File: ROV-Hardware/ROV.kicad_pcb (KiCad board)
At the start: 2 copper layers, 104 x 104 mm, 32 parts, among them J1 T-block, J2 T-block, J3 Screw_Terminal_01x04, SW1 switch, U1 LM7812, U2 LM7805, U3 ESP32-S3-DEVKITC-1-N8R2, U4 MPU6050, U5 ZK-BM1, U6 ZK-BM1, U7 ZK-BM1, U8 A4988, U9 GY-MS5837

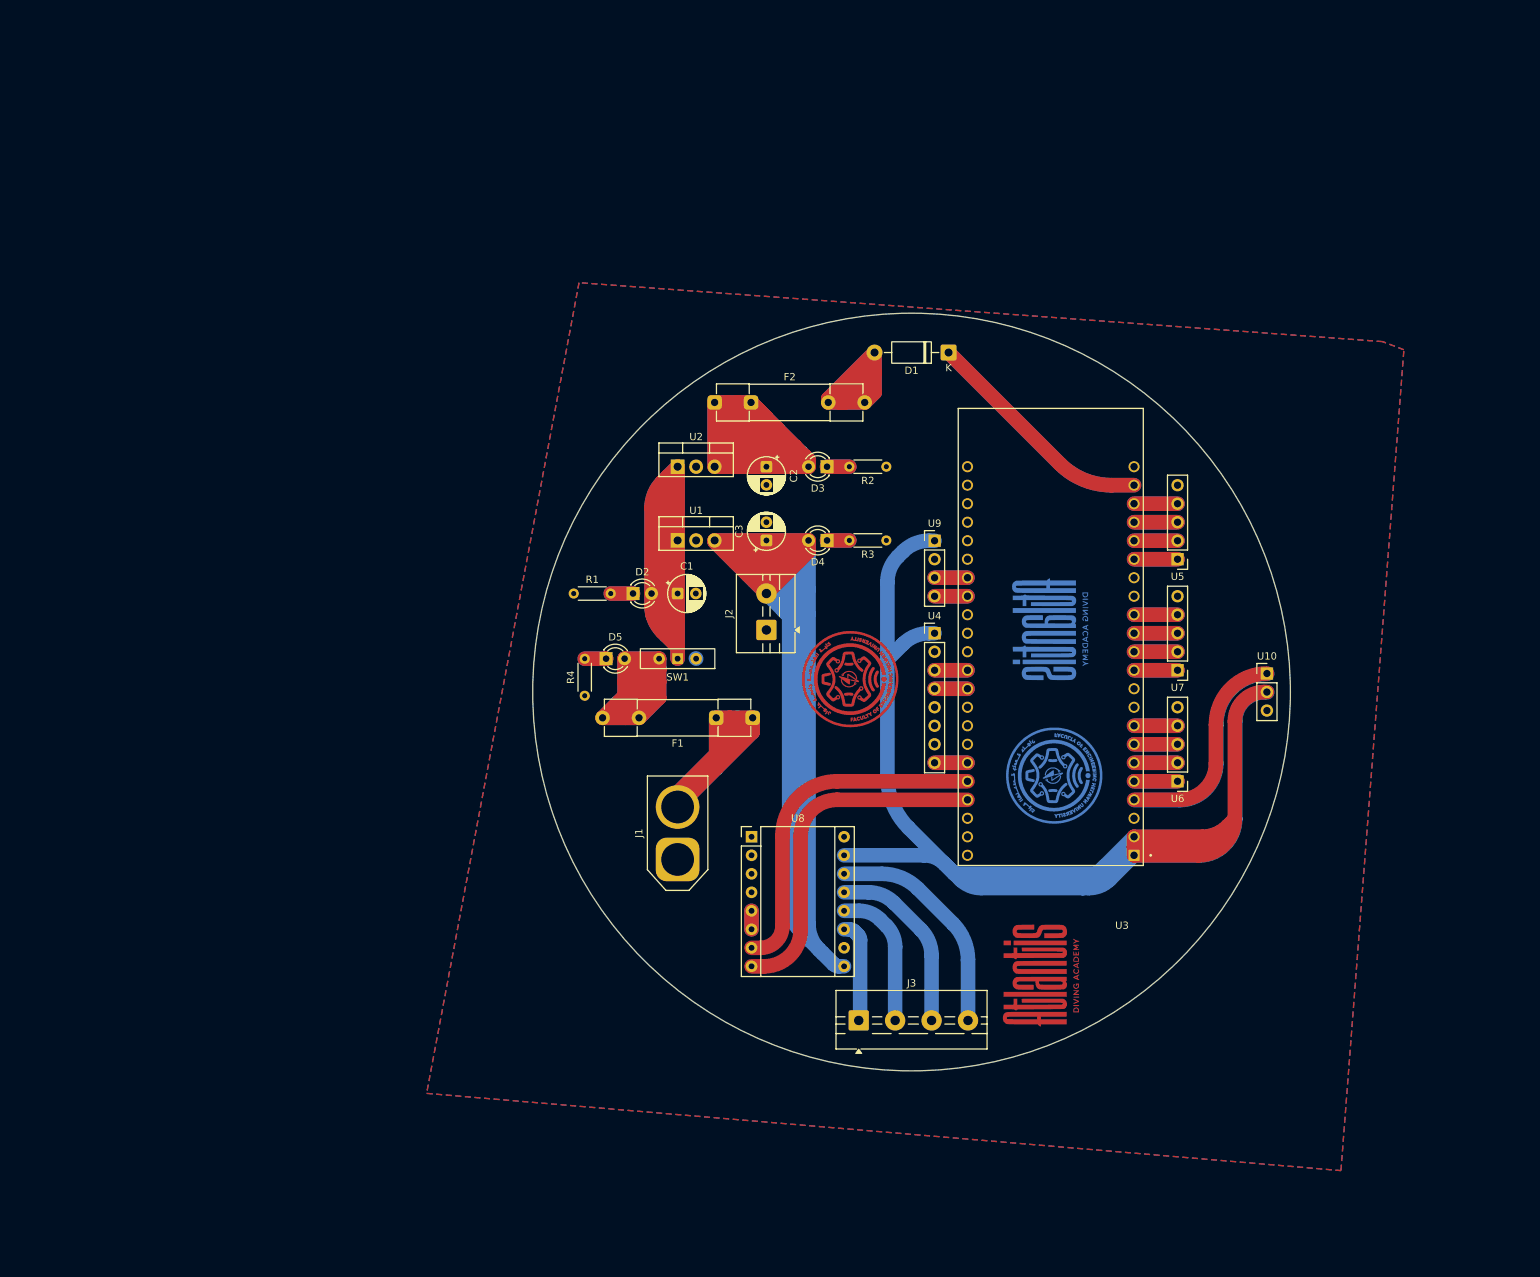
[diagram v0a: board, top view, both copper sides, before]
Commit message: hight current
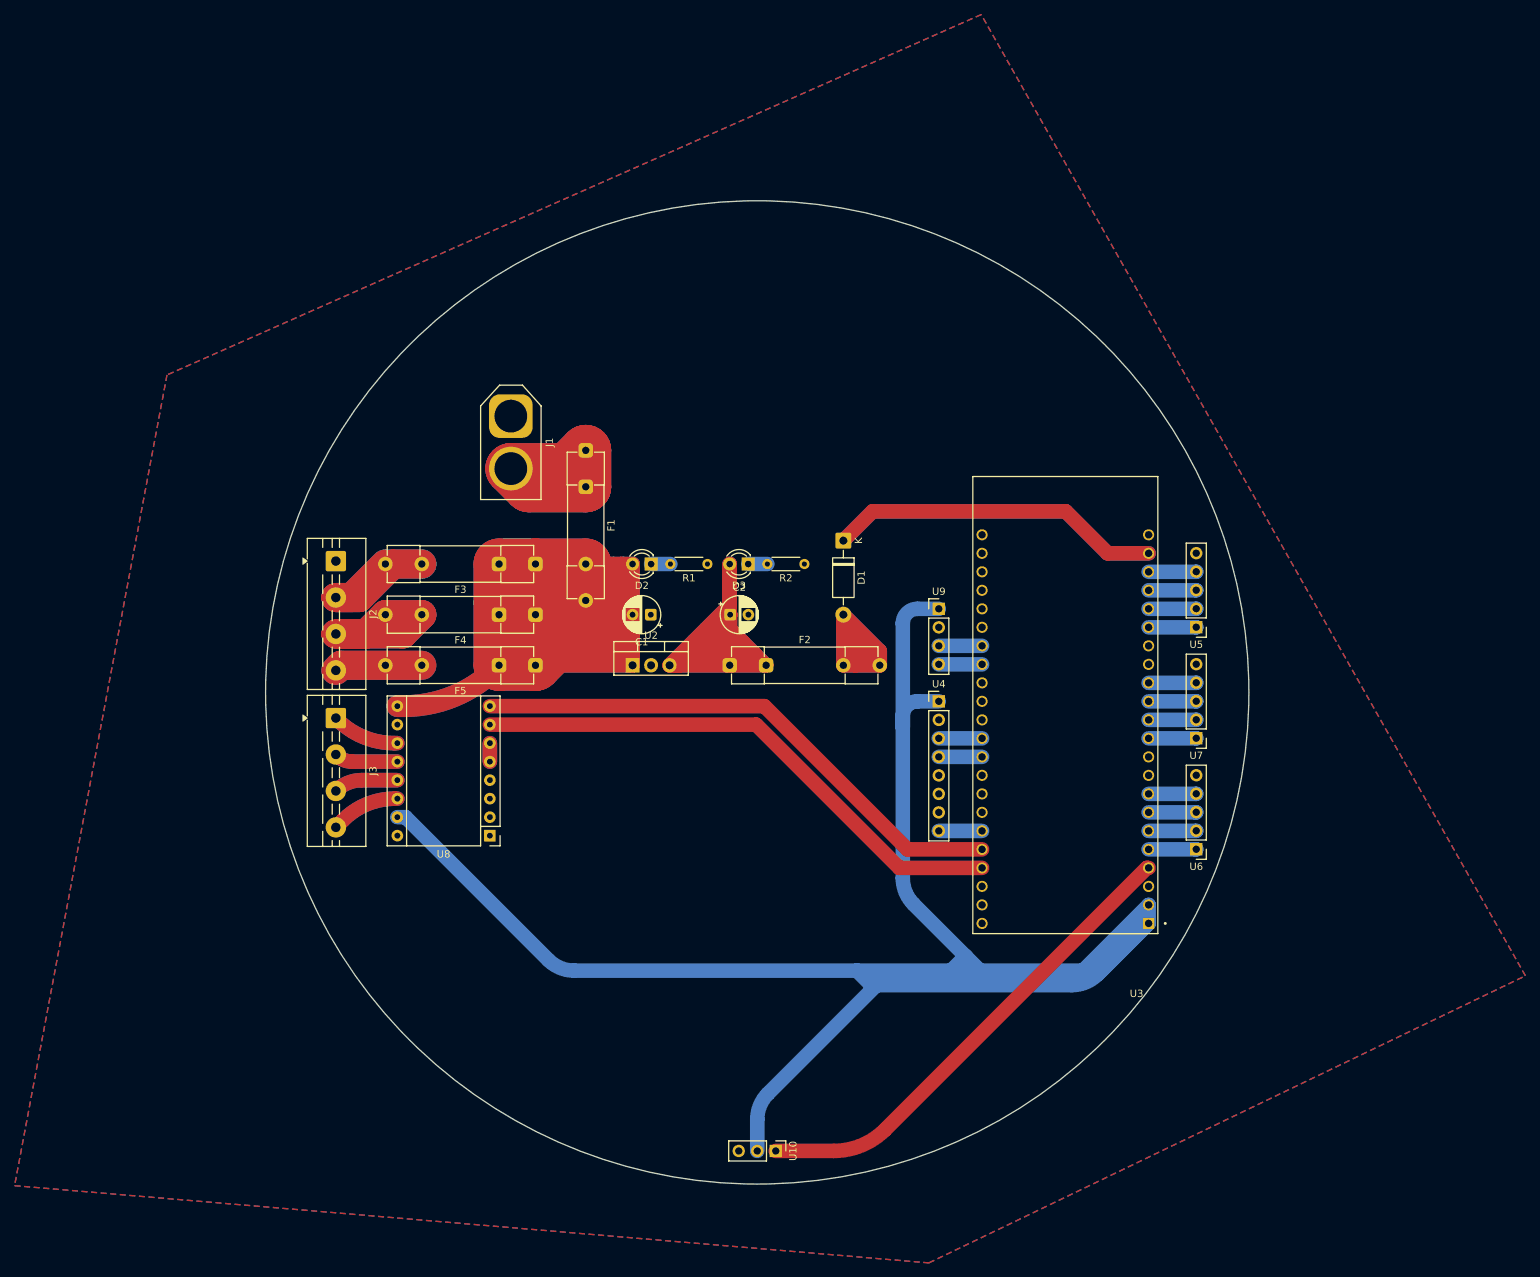
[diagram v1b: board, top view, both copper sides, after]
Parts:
- removed C3: capacitor, Capacitor_THT:CP_Radial_D5.0mm_P2.50mm
- removed D4, D5: LED, LED_THT:LED_D3.0mm
- removed G*** (x2): LOGO, logo:englogo4
- removed G*** (x2): LOGO, logo:logo7
- removed R3, R4: R, Resistor_THT:R_Axial_DIN0204_L3.6mm_D1.6mm_P5.08mm_Horizontal
- removed SW1: switch, Button_Switch_THT:SW_Slide-03_Wuerth-WS-SLTV_10x2.5x6.4_P2.54mm
- removed U1: LM7812, Package_TO_SOT_THT:TO-220-3_Vertical
- added F3: fuse, Fuse:Fuseholder_Clip-5x20mm_Schurter_CQM_Inline_P20.60x5.00mm_D1.00mm_Horizontal, F.Cu at (97.8, 81.5)
- added F4: fuse, Fuse:Fuseholder_Clip-5x20mm_Schurter_CQM_Inline_P20.60x5.00mm_D1.00mm_Horizontal, F.Cu at (97.8, 88.5)
- added F5: fuse, Fuse:Fuseholder_Clip-5x20mm_Schurter_CQM_Inline_P20.60x5.00mm_D1.00mm_Horizontal, F.Cu at (97.8, 95.4)
- J2: value T-block -> Screw_Terminal_01x04; footprint TerminalBlock:TerminalBlock_MaiXu_MX126-5.0-02P_1x02_P5.00mm -> TerminalBlock:TerminalBlock_MaiXu_MX126-5.0-04P_1x04_P5.00mm
- moved U10 94.0 mm to (130.8, 162.1), turned to -90 degrees
- moved J3 82.9 mm to (70.4, 102.6), turned to -90 degrees
- moved J1 65.0 mm to (94.4, 61.2), turned to -90 degrees
- moved J2 59.9 mm to (70.4, 81.1), turned to -90 degrees
- moved F1 43.3 mm to (104.7, 65.9), turned to -90 degrees
- moved F2 36.1 mm to (124.5, 95.4)
- moved U8 35.9 mm to (91.5, 118.8), turned to 180 degrees
- moved D1 29.6 mm to (140.1, 78.3), turned to -90 degrees
- moved U2 28.0 mm to (111.1, 95.4)
- moved C2 20.9 mm to (124.5, 88.5), turned to 0 degrees
- moved R1 18.8 mm to (121.4, 81.5), turned to 180 degrees
- moved R2 17.5 mm to (134.7, 81.5)
- moved D3 17.2 mm to (127.0, 81.5)
- moved U6 9.68 mm to (188.5, 120.7)
- moved U5 9.68 mm to (188.5, 90.2)
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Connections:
- C1 pad 1: Net-(D2-A) -> GNDREF
- C1 pad 2: GNDREF -> Net-(D2-A)
- F1 pad 2: Net-(D5-A) -> Net-(D2-A)
- J2 pad 2: Net-(D4-A) -> Net-(J2-Pin_2)
- U8 pad 7: Net-(U3-GPIO2) -> Net-(U3-GPIO1)
- U8 pad 8: Net-(U3-GPIO1) -> Net-(U3-GPIO2)
- U8 pad 9: Net-(D4-A) -> Net-(D2-A)
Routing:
- net Net-(D4-A): track 346.6 -> 0.00 mm
- net Net-(D2-A): track 217.1 -> 370.0 mm
- net Net-(D5-A): track 100.5 -> 0.00 mm
- net Net-(J2-Pin_2): track 0.00 -> 49.8 mm
- net Net-(J2-Pin_3): track 0.00 -> 47.4 mm
- net +12V: track 104.7 -> 58.8 mm
- net Net-(D3-A): track 186.7 -> 156.9 mm
- net Net-(U3-GPIO2): track 47.6 -> 75.7 mm
- net Net-(U3-GPIO1): track 47.8 -> 75.7 mm
- net +5V: track 65.0 -> 91.9 mm
- net Net-(J2-Pin_4): track 0.00 -> 24.2 mm
- net Net-(J3-Pin_4): track 31.2 -> 19.2 mm
- net Net-(J3-Pin_3): track 25.3 -> 17.6 mm
- net Net-(D1-A): track 59.3 -> 66.4 mm
- net Net-(U10-S): track 59.9 -> 66.8 mm
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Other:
- board size 104 x 104 mm -> 135 x 135 mm
